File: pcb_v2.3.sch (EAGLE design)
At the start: 57 parts, among them J1 PJ301_THONKICONN6, J2 PJ301_THONKICONN6, J3 PJ301_THONKICONN6, J4 PJ301_THONKICONN6, U1 MCP6004, U2 TL074_SMD, U5 TL074

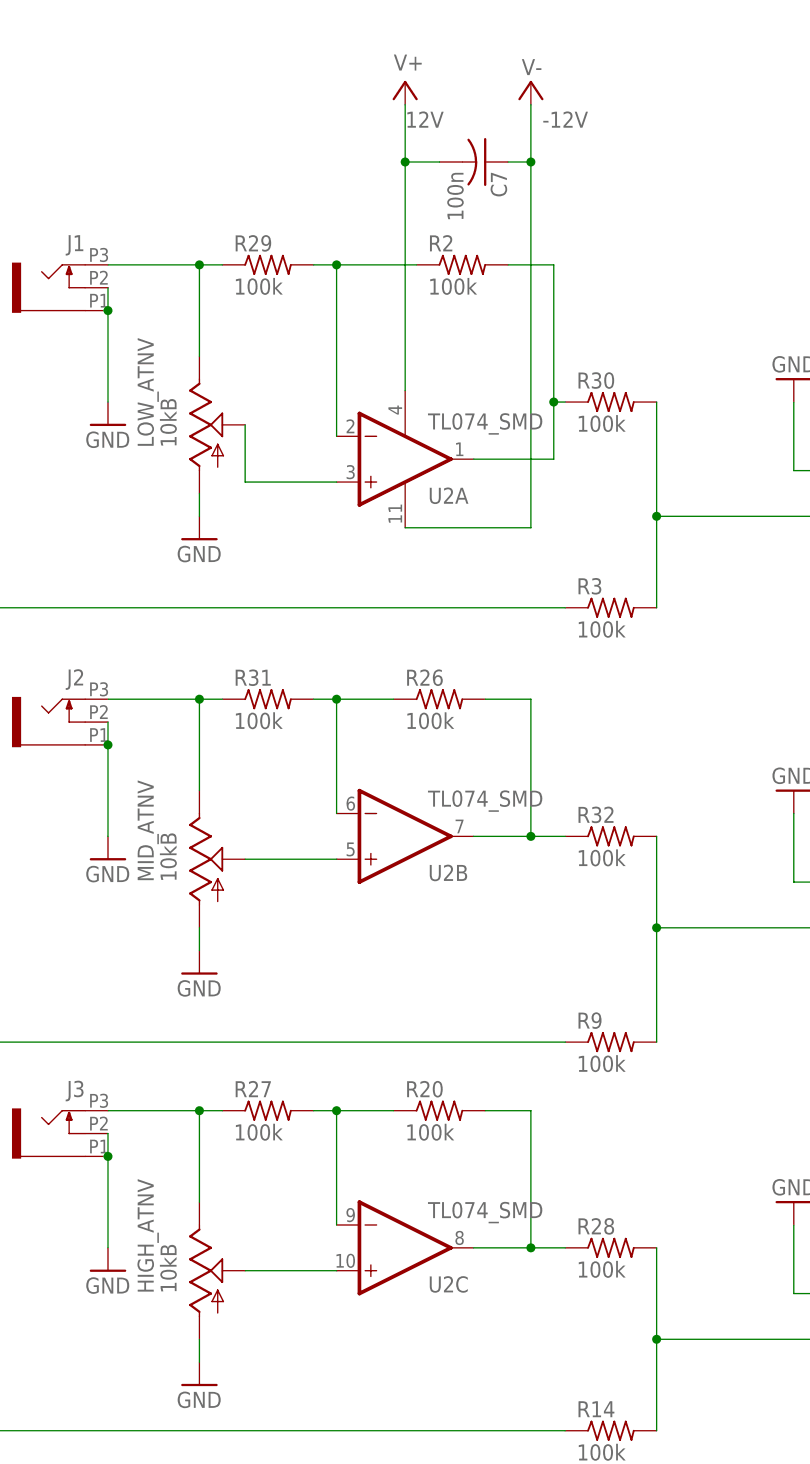
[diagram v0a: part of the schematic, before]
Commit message: new board layout
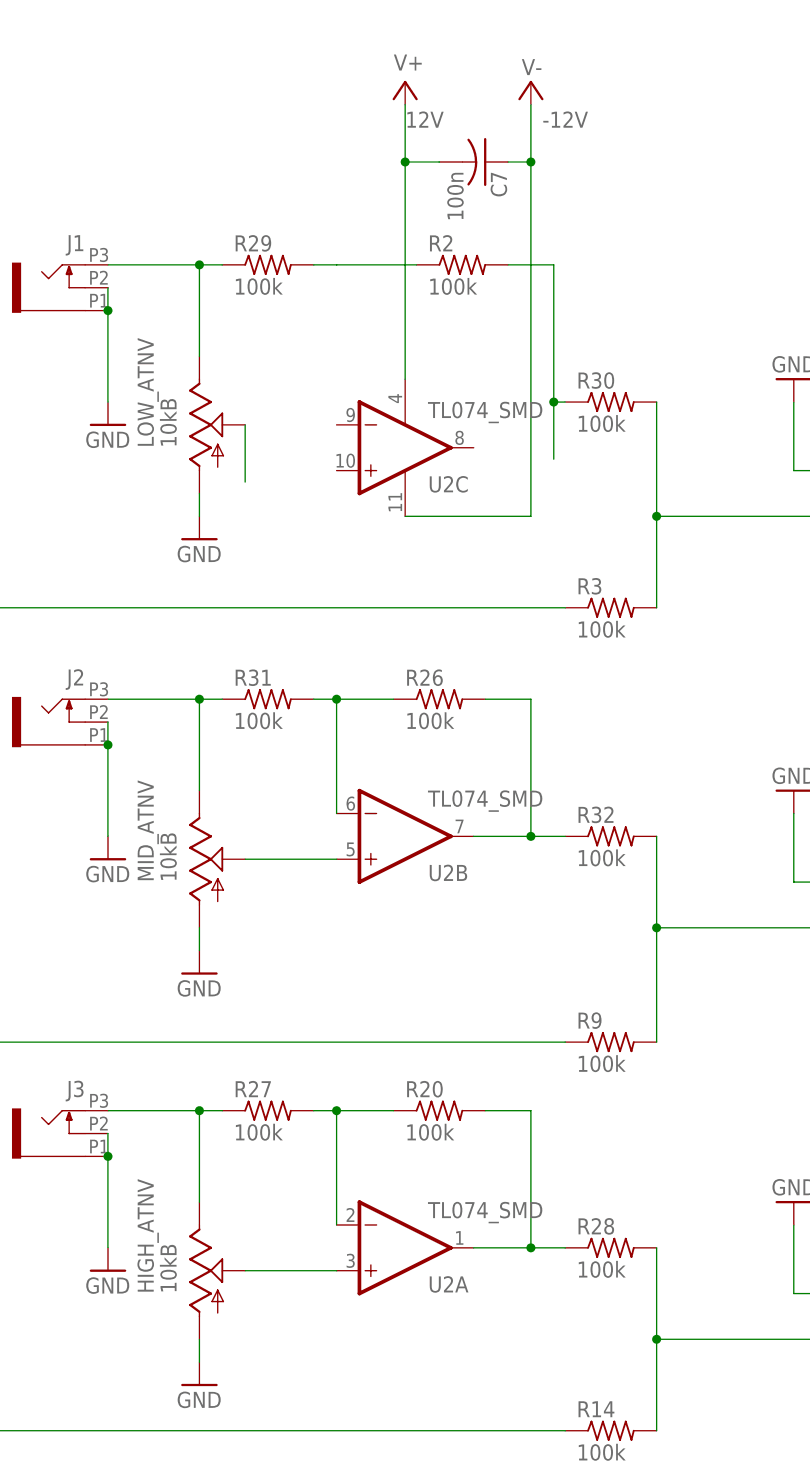
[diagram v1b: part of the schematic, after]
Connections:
- net N$14 renamed HIGH_SUM_FDBK
- net N$19 renamed MOD_SUM_FDBK
- net N$4 renamed LOW_SUM_FDBK
- net N$9 renamed MID_SUM_FDBK
- net N$1: no longer U2A.-IN
- net N$10: no longer U2A.+IN
- net N$13: now also U2A.OUT; no longer U2C.OUT
- net N$3: no longer U2A.OUT
- net N$6: now also U2A.-IN; no longer U2C.-IN
- net N$7: now also U2A.+IN; no longer U2C.+IN
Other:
- moved on the sheet: U2A, U2C
